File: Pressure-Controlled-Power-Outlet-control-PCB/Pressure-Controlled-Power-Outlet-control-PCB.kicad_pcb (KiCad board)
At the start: 4 copper layers, 99.1 x 82.5 mm, 25 parts, among them J1 Analog water pressure sensor 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, J2 1017514, K1 T9GV5L24-24, K2 T9GV5L24-24, Q1 2N3906, Q2 IRF540N, Q3 IRF540N, Q4 2N3906, U1 Pico, U2 LM324, U3 LF50_TO220

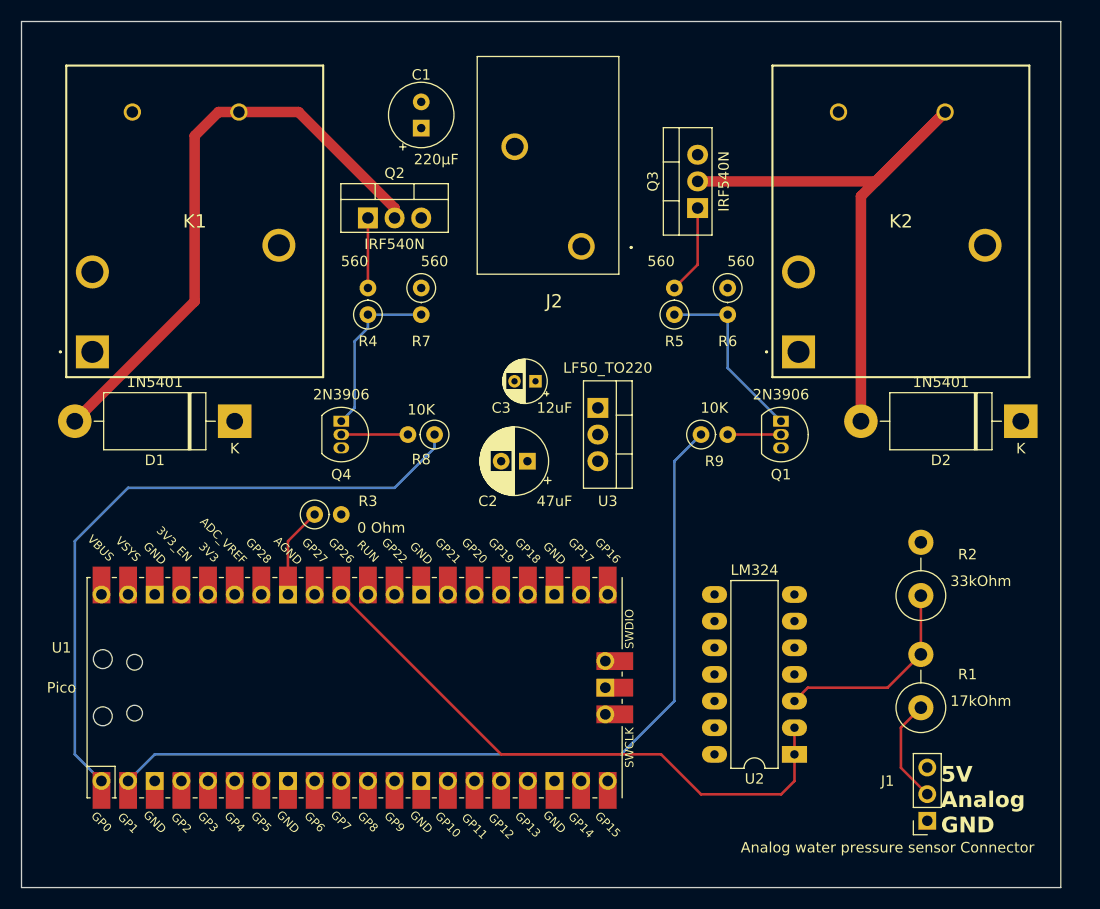
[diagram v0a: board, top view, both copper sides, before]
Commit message: should be done need to review the board to ensure everything is good
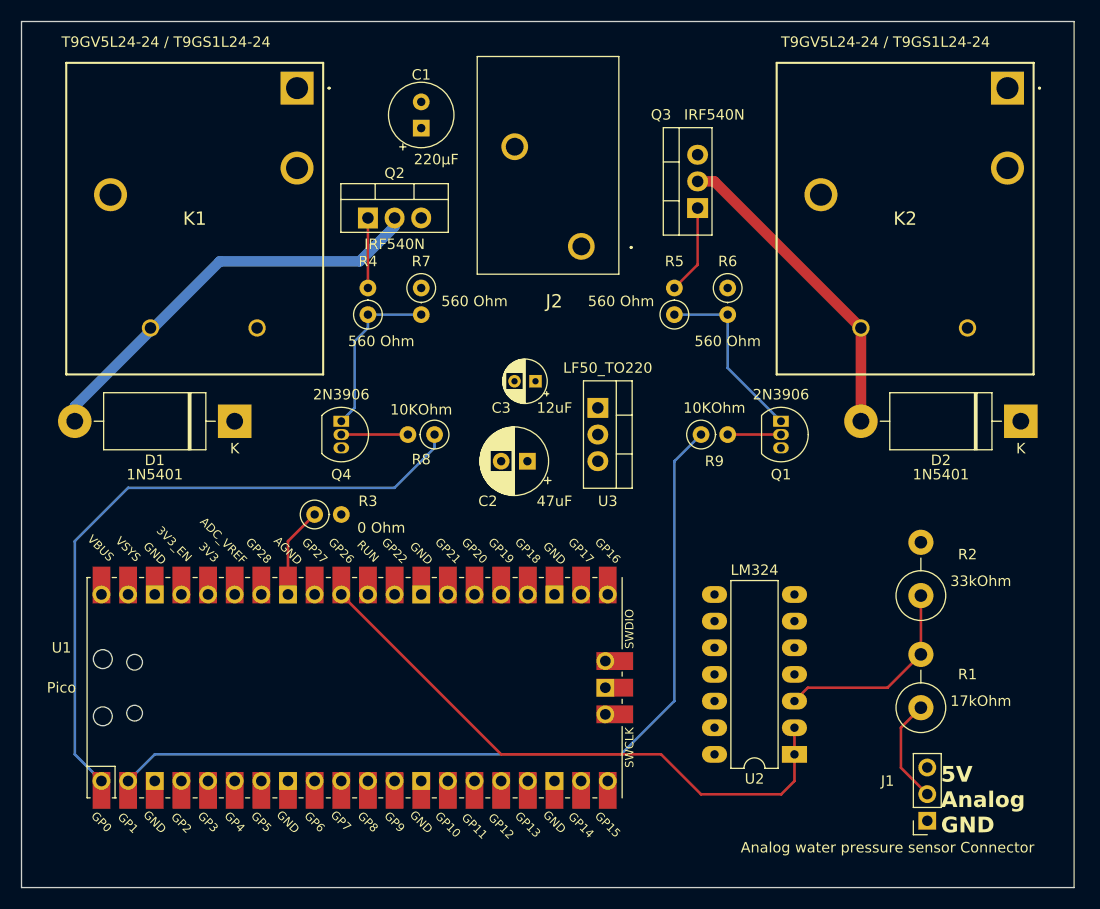
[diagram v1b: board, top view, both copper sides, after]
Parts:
- R4, R5, R6, R7: value 560 -> 560 Ohm
- R8, R9: value 10K -> 10KOhm
- moved K2 32.1 mm to (180.3, 72.4), turned to 180 degrees
- moved K1 31.8 mm to (112.6, 72.4), turned to 180 degrees
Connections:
- U1 pad 35: /ADC_Ref -> unconnected-(U1-ADC_VREF-Pad35)
- U2 pad 11: (no net) -> GND
- U2 pad 4: (no net) -> +5V
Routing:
- net Net-(D2-A): track 58.7 -> 30.2 mm
- net Net-(D1-A): track 56.7 -> 39.8 mm
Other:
- board size 99.1 x 82.5 mm -> 100.3 x 82.5 mm
- board text added: "T9GV5L24-24 / T9GS1L24-24"
